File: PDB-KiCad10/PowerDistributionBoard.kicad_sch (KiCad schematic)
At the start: 14 parts, among them U1 XL4016, U3 AMS1117

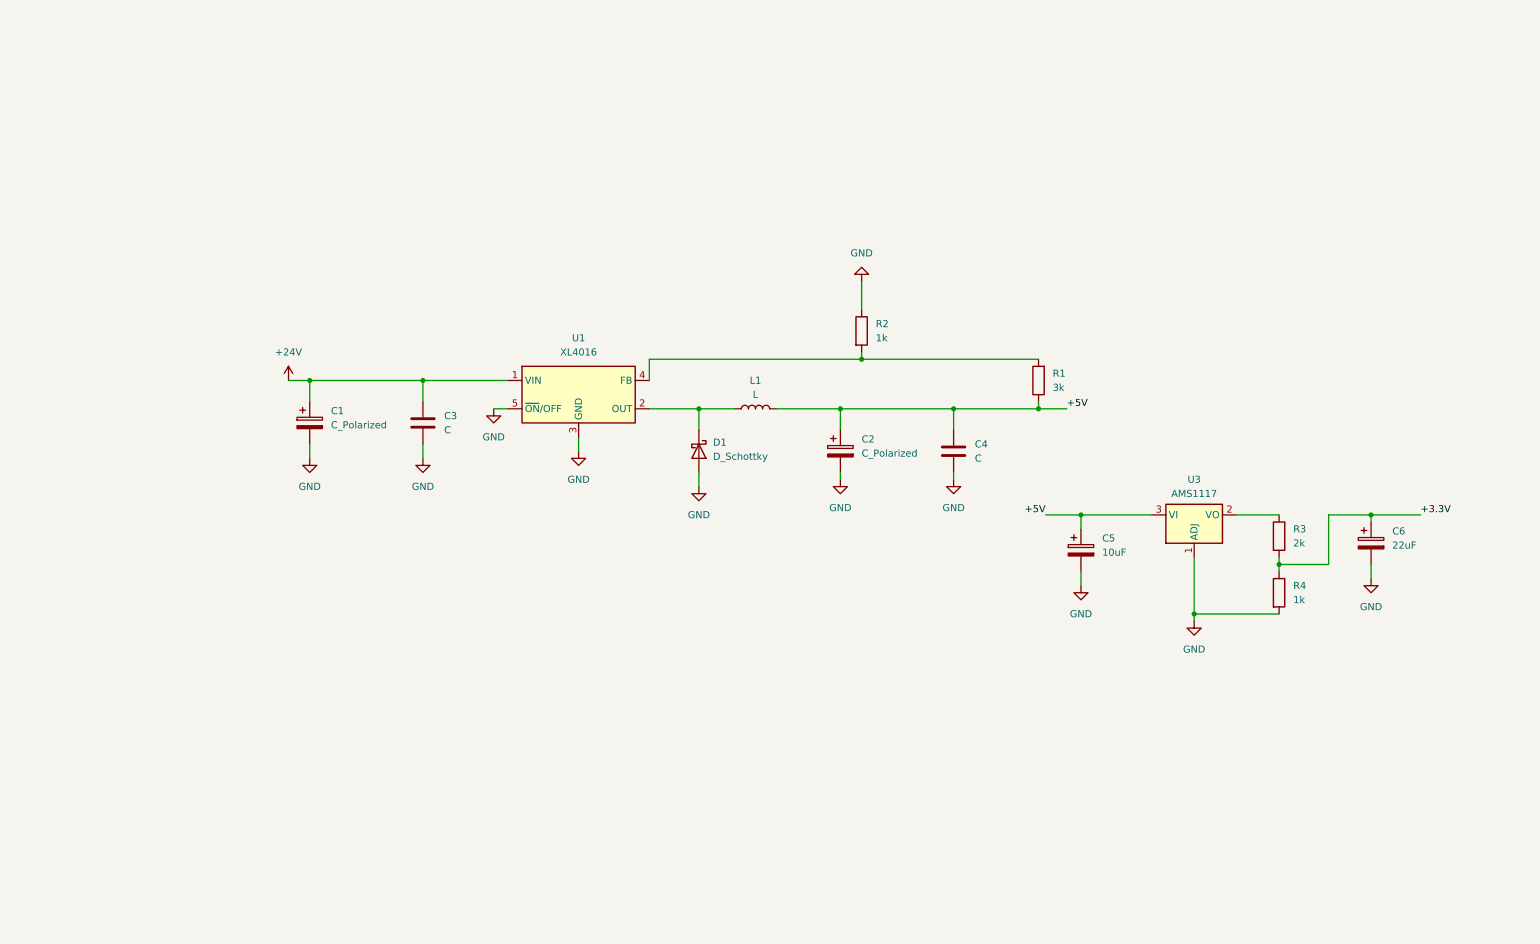
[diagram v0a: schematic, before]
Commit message: Upgraded the schematic
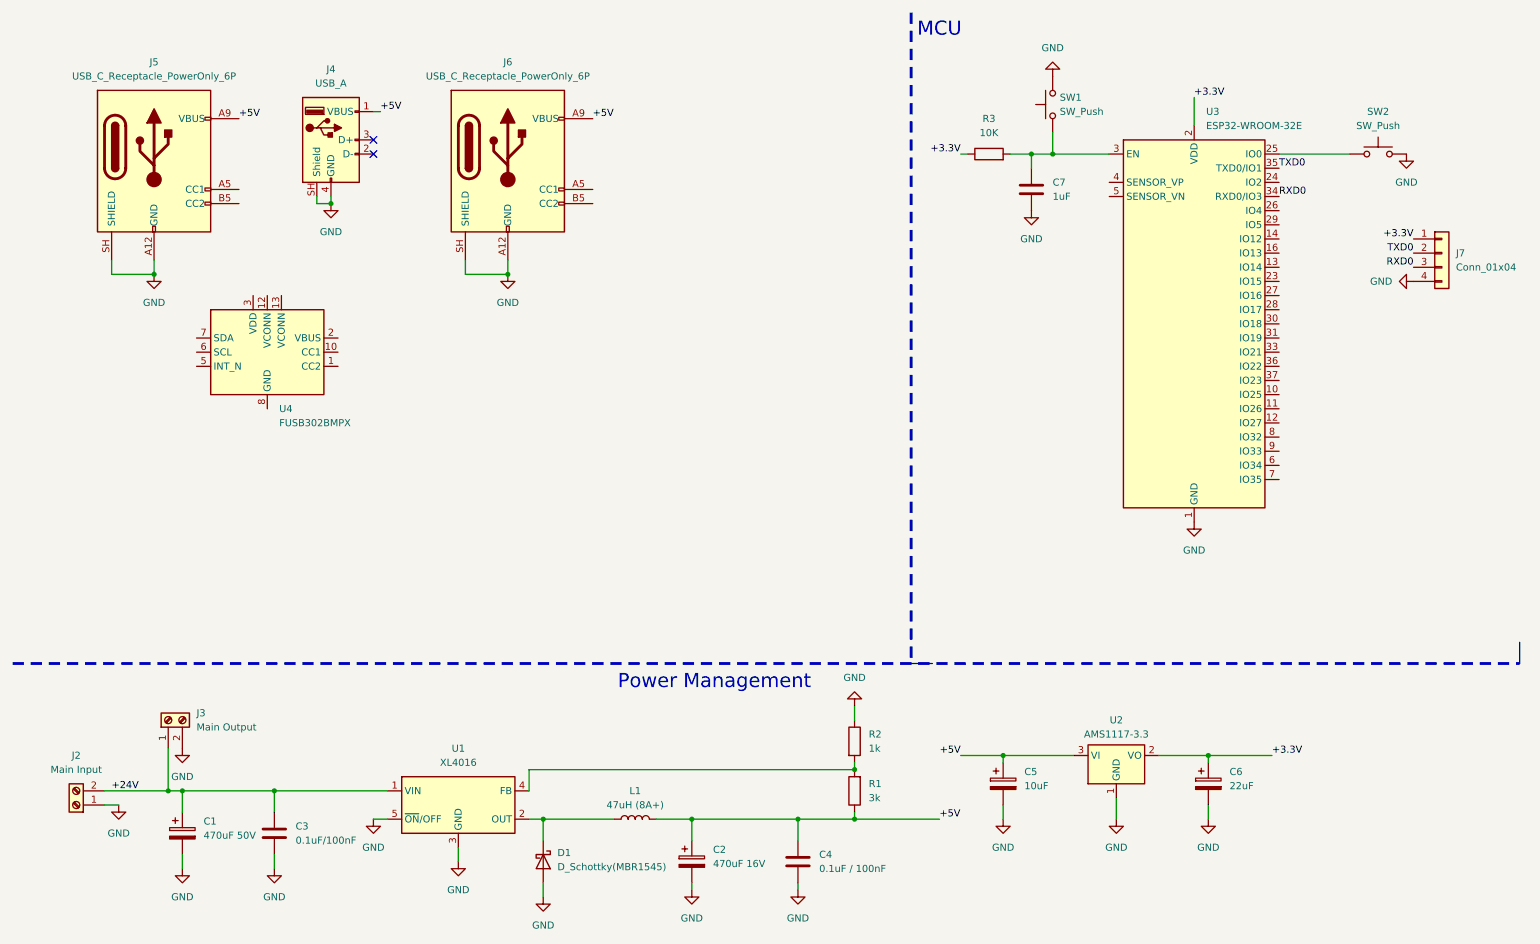
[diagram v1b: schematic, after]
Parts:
- removed R4: 1k, symbol Device:R
- removed U3: AMS1117, Package_TO_SOT_SMD:SOT-223-3_TabPin2, symbol Regulator_Linear:AMS1117
- added C7: 1uF, symbol Device:C
- added J2: Main Input, symbol Connector:Screw_Terminal_01x02
- added J3: Main Output, symbol Connector:Screw_Terminal_01x02
- added J4: USB_A, Connector_USB:USB_A_Molex_67643_Horizontal, symbol Connector:USB_A
- added J5, J6: USB_C_Receptacle_PowerOnly_6P, symbol Connector:USB_C_Receptacle_PowerOnly_6P
- added J7: Conn_01x04, symbol Connector_Generic:Conn_01x04
- added SW1, SW2: SW_Push, symbol Switch:SW_Push
- added U2: AMS1117-3.3, Package_TO_SOT_SMD:SOT-223-3_TabPin2, symbol Regulator_Linear:AMS1117-3.3
- added U3: ESP32-WROOM-32E, RF_Module:ESP32-WROOM-32D, symbol RF_Module:ESP32-WROOM-32E
- added U4: FUSB302BMPX, Package_DFN_QFN:WQFN-14-1EP_2.5x2.5mm_P0.5mm_EP1.45x1.45mm, symbol Interface_USB:FUSB302BMPX
- C1: value C_Polarized -> 470uF 50V
- C2: value C_Polarized -> 470uF 16V
- C3: value C -> 0.1uF/100nF
- C4: value C -> 0.1uF / 100nF
- D1: value D_Schottky -> D_Schottky(MBR1545)
- L1: value L -> 47uH (8A+)
- R3: value 2k -> 10K
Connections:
- net +24V: now also J2.2 (Pin_2), J3.1 (Pin_1)
- net +3.3V: now also R3.1, J7.1 (Pin_1), U2.2 (VO), U3.2 (VDD); no longer R3.2
- net +5V: now also J4.1 (VBUS), J5.A9 (VBUS), J5.B9 (VBUS), J6.A9 (VBUS), J6.B9 (VBUS), U2.3 (VI)
- net GND: now also C7.2, J2.1 (Pin_1), J3.2 (Pin_2), J4.4 (GND), J4.SH (Shield), J5.A12 (GND), J5.B12 (GND), J5.SH (SHIELD), J6.A12 (GND), J6.B12 (GND), J6.SH (SHIELD), J7.4 (Pin_4), SW1.2, SW2.2, U2.1 (GND), U3.1 (GND), U3.15 (GND), U3.38 (GND), U3.39 (GND)
- new net: C7.1, R3.2, SW1.1, U3.3 (EN)
- new net: U4.1 (CC2), U4.14 (CC2)
- new net: U4.10 (CC1), U4.11 (CC1)
- new net: U4.15 (GND), U4.8 (GND), U4.9 (GND)
- new net: U4.3 (VDD), U4.4 (VDD)
- new net: SW2.1, U3.25 (IO0)
- new net RXD0: J7.3 (Pin_3), U3.34 (RXD0/IO3)
- new net TXD0: J7.2 (Pin_2), U3.35 (TXD0/IO1)
- no-connect marks 0 -> 2
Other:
- note added: "MCU"
- note added: "Power Management"
- moved on the sheet: C1, C2, C3, C4, C5, C6, D1, L1, R1, R2, U1
